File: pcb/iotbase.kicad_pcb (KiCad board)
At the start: 2 copper layers, 43.2 x 48.9 mm, 38 parts, among them J1 USB_C_Receptacle_USB2.0, J2 RCWL-0516, J3 HSPI, J4 VSPI, U1 HDC1080, U2 AMS1117-3.3, U3 Connector_I2C, U4 Connector_I2C, U5 ESP32-WROOM-E, U6 Connector_IoT_GPIO, U7 Connector_ESProg

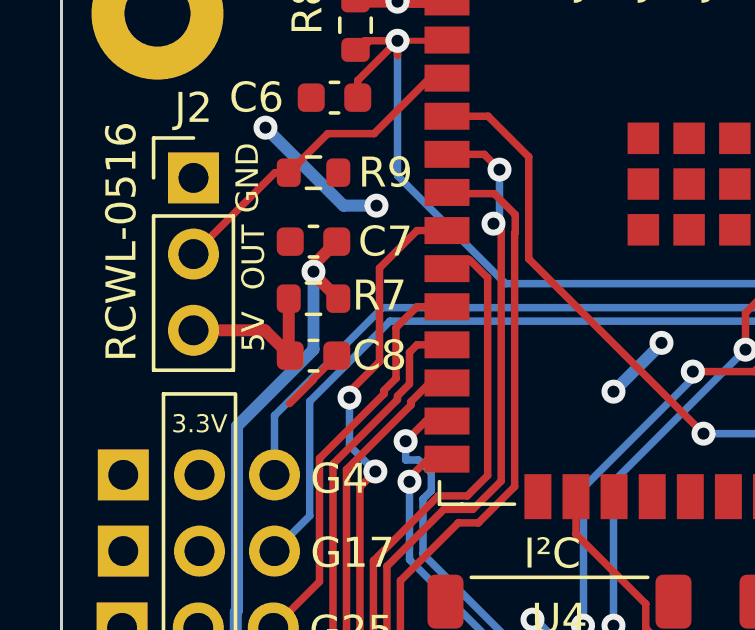
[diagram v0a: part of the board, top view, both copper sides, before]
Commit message: release rev. 0.2
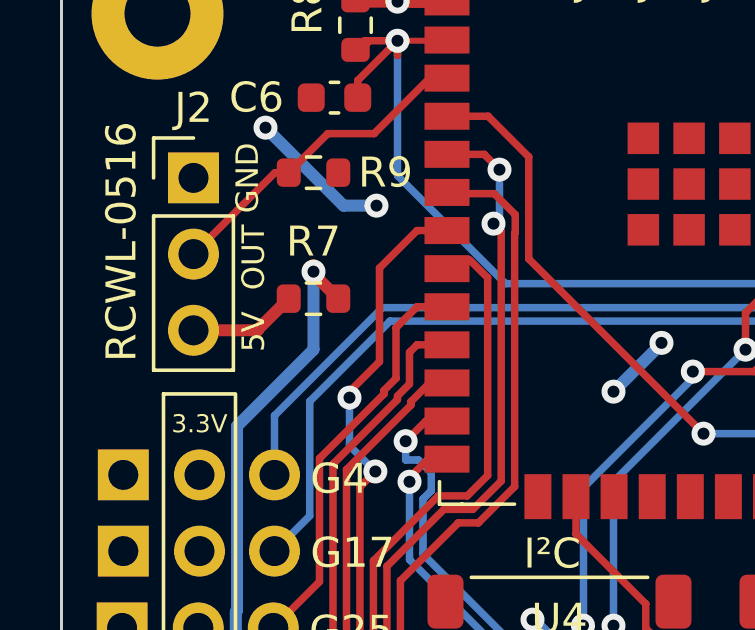
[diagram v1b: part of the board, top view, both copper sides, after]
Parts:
- removed C7, C8: 1000uF, Capacitor_SMD:C_0603_1608Metric
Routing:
- net GND: track 47.5 -> 45.2 mm
- net Net-(J2-Pad1): track 5.50 -> 3.63 mm
- net VBUS: track 87.2 -> 86.1 mm
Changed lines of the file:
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@@
   (net 51 "unconnected-(U1-Pad4)")
   (net 52 "unconnected-(U1-Pad7)")
-  (net 53 "Net-(C8-Pad1)")
+  (net 53 "Net-(J2-Pad1)")
   (footprint "Espressif:ESP32-WROOM-32E" (layer "F.Cu")
     (at 120.2 98.55)
@@
     )
   )
-  (footprint "Capacitor_SMD:C_0603_1608Metric" (layer "F.Cu")
-    (at 107 100.8 180)
-    (descr "Capacitor SMD 0603 (1608 Metric), square (rectangular) end terminal, IPC_7351 nominal, (Body size source: IPC-SM-782 page 76, https://www.pcb-3d.com/wordpress/wp-content/uploads/ipc-sm-782a_amendment_1_and_2.pdf), generated with kicad-footprint-generator")
-    (tags "capacitor")
-    (property "Sheetfile" "iotbase.kicad_sch")
-    (property "Sheetname" "")
-    (attr smd)
-    (fp_text reference "C7" (at -2.4 0) (layer "F.SilkS")
-      (effects (font (size 1 1) (thickness 0.15)))
-    )
-    (fp_text value "1000uF" (at 0 1.43) (layer "F.Fab")
-      (effects (font (size 1 1) (thickness 0.15)))
-    )
-    (fp_text user "${REFERENCE}" (at 0 0) (layer "F.Fab")
-      (effects (font (size 0.4 0.4) (thickness 0.06)))
-    )
-    (fp_line (start -0.14058 0.51) (end 0.14058 0.51) (layer "F.SilkS") (width 0.12))
-    (fp_line (start -0.14058 -0.51) (end 0.14058 -0.51) (layer "F.SilkS") (width 0.12))
-    (fp_line (start 1.48 0.73) (end -1.48 0.73) (layer "F.CrtYd") (width 0.05))
-    (fp_line (start -1.48 0.73) (end -1.48 -0.73) (layer "F.CrtYd") (width 0.05))
-    (fp_line (start 1.48 -0.73) (end 1.48 0.73) (layer "F.CrtYd") (width 0.05))
-    (fp_line (start -1.48 -0.73) (end 1.48 -0.73) (layer "F.CrtYd") (width 0.05))
-    (fp_line (start -0.8 -0.4) (end 0.8 -0.4) (layer "F.Fab") (width 0.1))
-    (fp_line (start 0.8 -0.4) (end 0.8 0.4) (layer "F.Fab") (width 0.1))
-    (fp_line (start 0.8 0.4) (end -0.8 0.4) (layer "F.Fab") (width 0.1))
-    (fp_line (start -0.8 0.4) (end -0.8 -0.4) (layer "F.Fab") (width 0.1))
-    (pad "1" smd roundrect (at -0.775 0 180) (size 0.9 0.95) (layers "F.Cu" "F.Paste" "F.Mask") (roundrect_rratio 0.25)
-      (net 1 "VBUS") (pintype "passive"))
-    (pad "2" smd roundrect (at 0.775 0 180) (size 0.9 0.95) (layers "F.Cu" "F.Paste" "F.Mask") (roundrect_rratio 0.25)
-      (net 2 "GND") (pintype "passive"))
-    (model "${KICAD6_3DMODEL_DIR}/Capacitor_SMD.3dshapes/C_0603_1608Metric.wrl"
-      (offset (xyz 0 0 0))
-      (scale (xyz 1 1 1))
-      (rotate (xyz 0 0 0))
-    )
-  )
   (footprint "Resistor_SMD:R_0603_1608Metric" (layer "F.Cu")
     (at 108.4 93.5834 -90)
@@
       (net 3 "RESET") (pintype "passive"))
     (model "${KICAD6_3DMODEL_DIR}/Resistor_SMD.3dshapes/R_0603_1608Metric.wrl"
-      (offset (xyz 0 0 0))
-      (scale (xyz 1 1 1))
-      (rotate (xyz 0 0 0))
-    )
-  )
-  (footprint "Capacitor_SMD:C_0603_1608Metric" (layer "F.Cu")
-    (at 107 104.6)
-    (descr "Capacitor SMD 0603 (1608 Metric), square (rectangular) end terminal, IPC_7351 nominal, (Body size source: IPC-SM-782 page 76, https://www.pcb-3d.com/wordpress/wp-content/uploads/ipc-sm-782a_amendment_1_and_2.pdf), generated with kicad-footprint-generator")
-    (tags "capacitor")
-    (property "Sheetfile" "iotbase.kicad_sch")
-    (property "Sheetname" "")
-    (attr smd)
-    (fp_text reference "C8" (at 2.2 0) (layer "F.SilkS")
-      (effects (font (size 1 1) (thickness 0.15)))
-    )
-    (fp_text value "1000uF" (at 0 1.43) (layer "F.Fab")
-      (effects (font (size 1 1) (thickness 0.15)))
-    )
-    (fp_text user "${REFERENCE}" (at 0 0) (layer "F.Fab")
-      (effects (font (size 0.4 0.4) (thickness 0.06)))
-    )
-    (fp_line (start -0.14058 -0.51) (end 0.14058 -0.51) (layer "F.SilkS") (width 0.12))
-    (fp_line (start -0.14058 0.51) (end 0.14058 0.51) (layer "F.SilkS") (width 0.12))
-    (fp_line (start -1.48 -0.73) (end 1.48 -0.73) (layer "F.CrtYd") (width 0.05))
-    (fp_line (start 1.48 0.73) (end -1.48 0.73) (layer "F.CrtYd") (width 0.05))
-    (fp_line (start 1.48 -0.73) (end 1.48 0.73) (layer "F.CrtYd") (width 0.05))
-    (fp_line (start -1.48 0.73) (end -1.48 -0.73) (layer "F.CrtYd") (width 0.05))
-    (fp_line (start 0.8 -0.4) (end 0.8 0.4) (layer "F.Fab") (width 0.1))
-    (fp_line (start 0.8 0.4) (end -0.8 0.4) (layer "F.Fab") (width 0.1))
-    (fp_line (start -0.8 -0.4) (end 0.8 -0.4) (layer "F.Fab") (width 0.1))
-    (fp_line (start -0.8 0.4) (end -0.8 -0.4) (layer "F.Fab") (width 0.1))
-    (pad "1" smd roundrect (at -0.775 0) (size 0.9 0.95) (layers "F.Cu" "F.Paste" "F.Mask") (roundrect_rratio 0.25)
-      (net 53 "Net-(C8-Pad1)") (pintype "passive"))
-    (pad "2" smd roundrect (at 0.775 0) (size 0.9 0.95) (layers "F.Cu" "F.Paste" "F.Mask") (roundrect_rratio 0.25)
-      (net 2 "GND") (pintype "passive"))
-    (model "${KICAD6_3DMODEL_DIR}/Capacitor_SMD.3dshapes/C_0603_1608Metric.wrl"
       (offset (xyz 0 0 0))
       (scale (xyz 1 1 1))
@@
     (property "Sheetname" "")
     (attr smd)
-    (fp_text reference "R7" (at -2.2 0.1) (layer "F.SilkS")
+    (fp_text reference "R7" (at 0 1.9) (layer "F.SilkS")
       (effects (font (size 1 1) (thickness 0.15)))
     )
@@
       (net 1 "VBUS") (pintype "passive"))
     (pad "2" smd roundrect (at 0.825 0 180) (size 0.8 0.95) (layers "F.Cu" "F.Paste" "F.Mask") (roundrect_rratio 0.25)
-      (net 53 "Net-(C8-Pad1)") (pintype "passive"))
+      (net 53 "Net-(J2-Pad1)") (pintype "passive"))
     (model "${KICAD6_3DMODEL_DIR}/Resistor_SMD.3dshapes/R_0603_1608Metric.wrl"
       (offset (xyz 0 0 0))
@@
     (fp_line (start -0.635 -1.27) (end 1.27 -1.27) (layer "F.Fab") (width 0.1))
     (pad "1" thru_hole oval (at 0 5.08) (size 1.7 1.7) (drill 1) (layers *.Cu *.Mask)
-      (net 53 "Net-(C8-Pad1)") (pinfunction "Pin_1") (pintype "passive"))
+      (net 53 "Net-(J2-Pad1)") (pinfunction "Pin_1") (pintype "passive"))
     (pad "2" thru_hole oval (at 0 2.54) (size 1.7 1.7) (drill 1) (layers *.Cu *.Mask)
       (net 27 "IO36") (pinfunction "Pin_2") (pintype "passive"))
@@
   (segment (start 117.83548 134.56452) (end 114.31452 134.56452) (width 0.4) (layer "F.Cu") (net 1))
   (segment (start 119.2 134.148073) (end 118.783553 134.56452) (width 0.4) (layer "F.Cu") (net 1))
-  (segment (start 107 101.575) (end 107.775 100.8) (width 0.4) (layer "F.Cu") (net 1))
   (segment (start 118.783553 134.56452) (end 117.83548 134.56452) (width 0.4) (layer "F.Cu") (net 1))
   (segment (start 113.8 122.4) (end 113.7 122.5) (width 0.4) (layer "F.Cu") (net 1))
@@
   (segment (start 134.8 116.67) (end 134.565179 116.904821) (width 0.25) (layer "F.Cu") (net 2))
   (segment (start 133.6 101.4) (end 133.6 105) (width 0.25) (layer "F.Cu") (net 2))
-  (segment (start 107.775 104.6) (end 106.97548 105.39952) (width 0.25) (layer "F.Cu") (net 2))
   (segment (start 133.6 105) (end 133.4 105.2) (width 0.25) (layer "F.Cu") (net 2))
-  (segment (start 106.97548 105.39952) (end 106.97548 105.42452) (width 0.25) (layer "F.Cu") (net 2))
   (segment (start 124.45 130.46) (end 124.625 130.285) (width 0.25) (layer "F.Cu") (net 2))
-  (segment (start 106.97548 105.42452) (end 106.2 106.2) (width 0.25) (layer "F.Cu") (net 2))
   (segment (start 134.565179 116.904821) (end 132.608837 116.904821) (width 0.25) (layer "F.Cu") (net 2))
   (segment (start 133.375 106.4) (end 133.375 105.225) (width 0.25) (layer "F.Cu") (net 2))
@@
   (segment (start 126.6 105.43) (end 126.6 103) (width 0.25) (layer "F.Cu") (net 13))
   (via (at 126.6 103) (size 0.8) (drill 0.4) (layers "F.Cu" "B.Cu") (net 13))
-  (segment (start 107.528228 104.771772) (end 107.528228 104.807547) (width 0.25) (layer "B.Cu") (net 13))
-  (segment (start 107.068045 105.231955) (end 105.7 106.6) (width 0.25) (layer "B.Cu") (net 13))
-  (segment (start 107.10382 105.231955) (end 107.068045 105.231955) (width 0.25) (layer "B.Cu") (net 13))
-  (segment (start 109.3 103) (end 107.528228 104.771772) (width 0.25) (layer "B.Cu") (net 13))
+  (segment (start 109.3 103) (end 105.7 106.6) (width 0.25) (layer "B.Cu") (net 13))
   (segment (start 105.7 106.6) (end 105.7 108.575) (width 0.25) (layer "B.Cu") (net 13))
-  (segment (start 107.528228 104.807547) (end 107.10382 105.231955) (width 0.25) (layer "B.Cu") (net 13))
   (segment (start 126.6 103) (end 109.3 103) (width 0.25) (layer "B.Cu") (net 13))
   (segment (start 111.425 137.45) (end 113.0125 137.45) (width 0.25) (layer "F.Cu") (net 14))
@@
   (segment (start 131.575 103.825) (end 129.89 105.51) (width 0.25) (layer "F.Cu") (net 41))
   (segment (start 131.575 96.6) (end 131.575 103.825) (width 0.25) (layer "F.Cu") (net 41))
-  (segment (start 105.38 103.755) (end 103 103.755) (width 0.4) (layer "F.Cu") (net 53))
-  (segment (start 106.175 102.7) (end 106.175 104.55) (width 0.4) (layer "F.Cu") (net 53))
-  (segment (start 106.175 104.55) (end 106.225 104.6) (width 0.25) (layer "F.Cu") (net 53))
-  (segment (start 106.225 104.6) (end 105.38 103.755) (width 0.4) (layer "F.Cu") (net 53))
+  (segment (start 105.145 103.755) (end 105.145 103.73) (width 0.4) (layer "F.Cu") (net 53))
+  (segment (start 105.145 103.73) (end 106.175 102.7) (width 0.4) (layer "F.Cu") (net 53))
+  (segment (start 105.145 103.755) (end 103 103.755) (width 0.4) (layer "F.Cu") (net 53))
   (zone (net 2) (net_name "GND") (layer "F.Cu") (hatch edge 0.508)
     (connect_pads (clearance 0.508))
@@
       66bf29d3-e872-4ea9-bbf4-cc6e9505dc01
       7df22e47-c5af-4da2-b6a2-8d776bdbfb48
-      7f20ddd7-877a-4d8f-91a1-342ccc274435
       864ca123-44ac-4bb5-a3d7-dc7822dbc294
       987c5747-6eb2-497e-a4eb-be9e6630b188
